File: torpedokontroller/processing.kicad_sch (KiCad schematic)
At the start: 33 parts, among them IC2 STM32C542CCT6, IC3 SN74AHCT1G125DCKR, J3 653104124022, J4 61300211021, J5 62701021621, J9 USB_C_Receptacle_USB2.0_16P, SW1 434123025826, SW2 434123025826, U5 WE-TVS-82400102, Y1 48 MHz

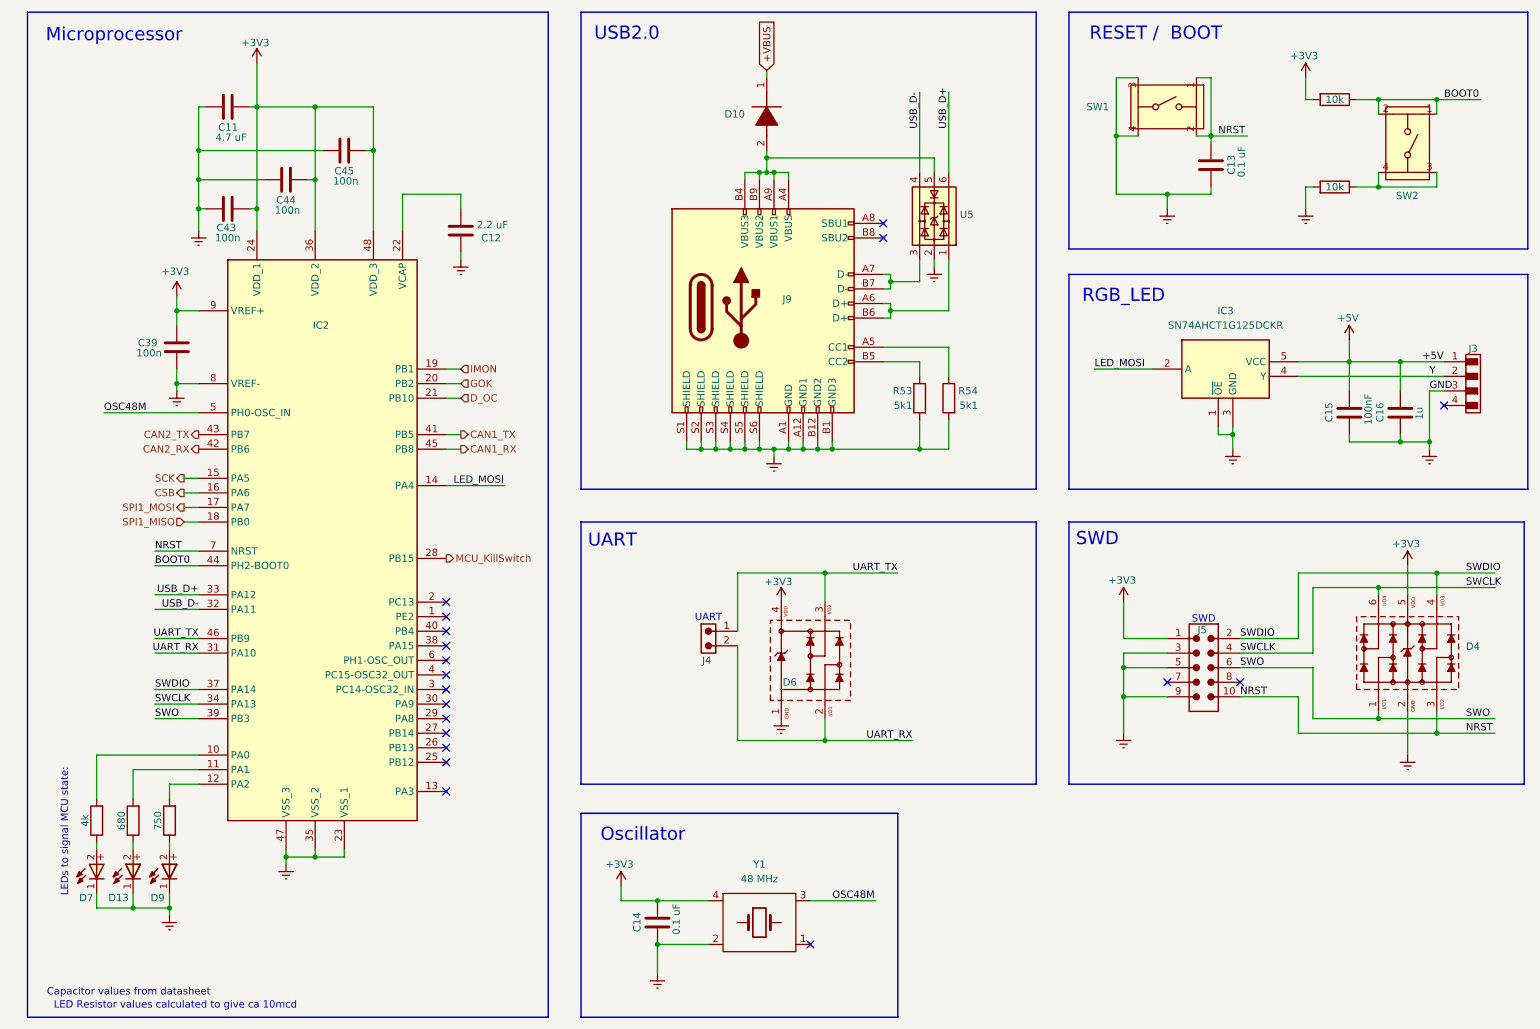
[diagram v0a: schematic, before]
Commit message: v 1.0
Ferdigish

CAN tvs-packages
Ground hook
Test pads
fixed some i/o issues
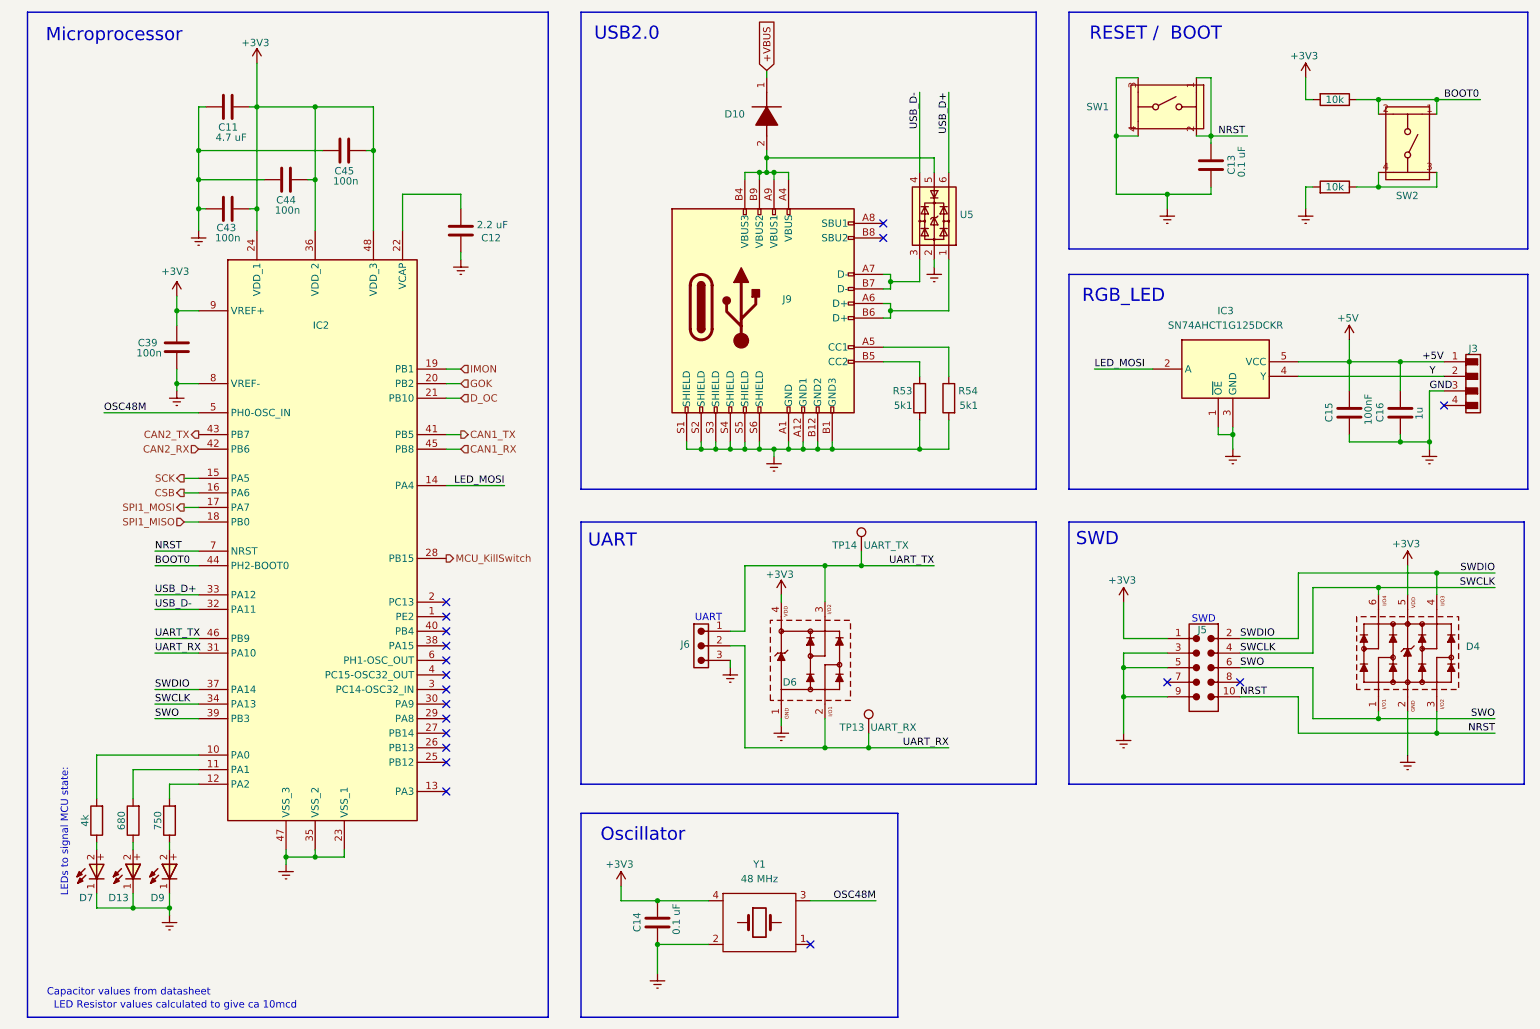
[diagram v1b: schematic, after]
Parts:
- removed J4: 61300211021, Connector_THT_Wurth:J_Wurth_WR-PHD_61300211021, symbol Connector_Wurth_WR-PHD:61300211021
- added J6: 61300311021, Connector_THT_Wurth:J_Wurth_WR-PHD_61300311021, symbol Connector_Wurth_WR-PHD:61300311021
- added TP13, TP14: TestPoint, TestPoint:TestPoint_Pad_D1.5mm, symbol Connector:TestPoint
- renumbered R to R1
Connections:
- net Earth: now also J6.3
- net UART_RX: now also J6.2, TP13.1
- net UART_TX: now also J6.1, TP14.1
